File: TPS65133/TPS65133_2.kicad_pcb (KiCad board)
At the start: 2 copper layers, 19.8 x 40.1 mm, 14 parts, among them IC1 TPS65133DPDR, J1 Conn_02x03_Odd_Even, J2 Conn_02x03_Odd_Even, J3 Conn_02x03_Odd_Even

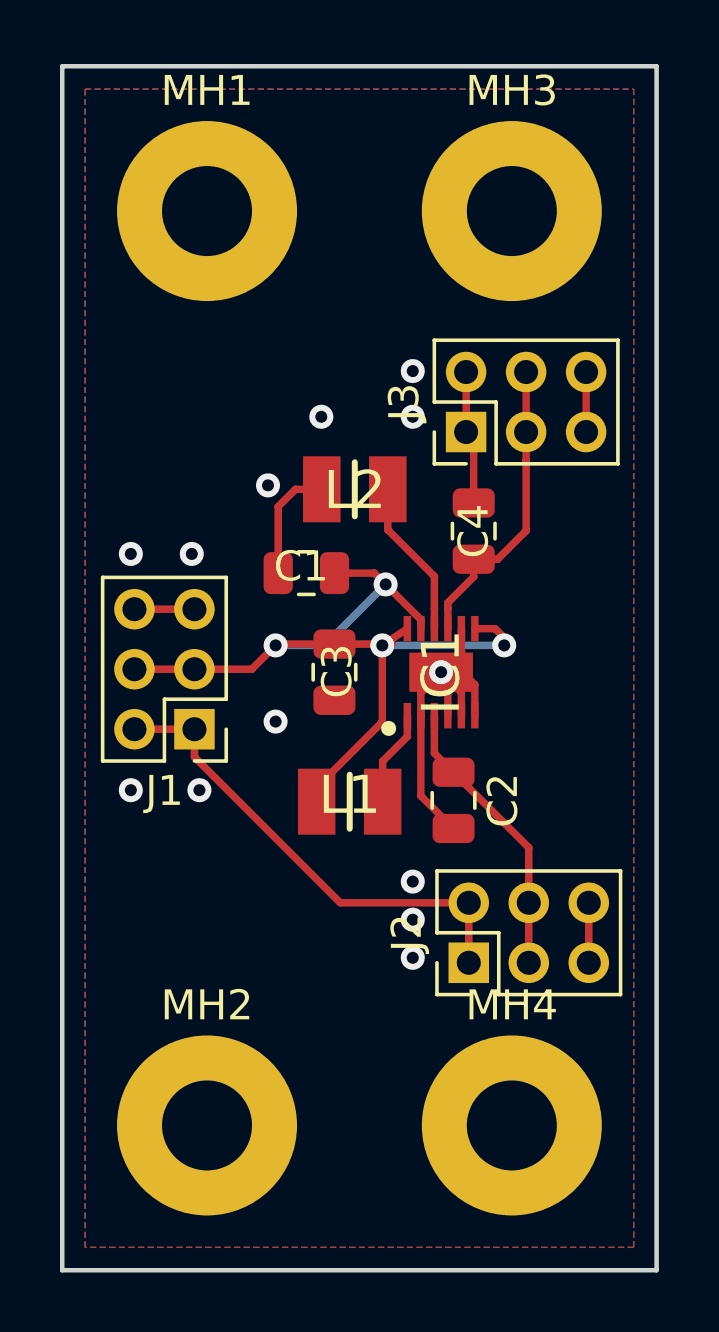
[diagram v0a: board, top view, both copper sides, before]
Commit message: TPS65133
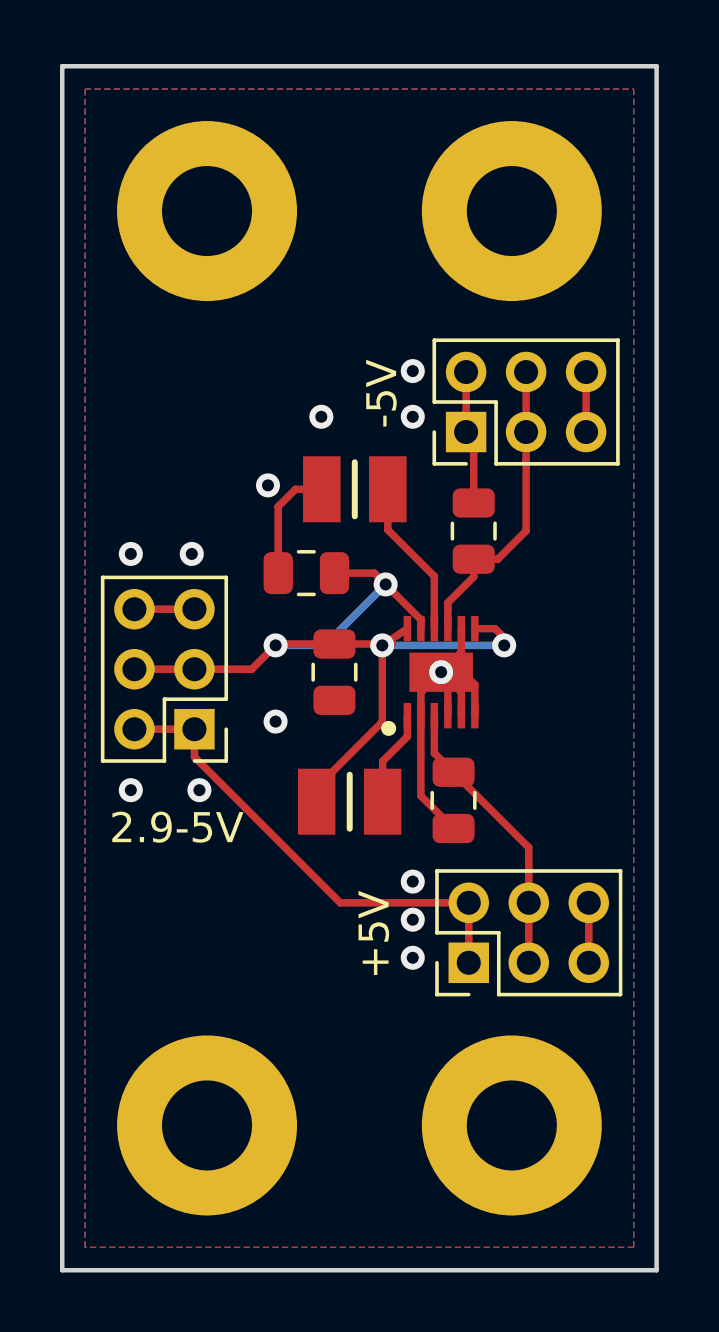
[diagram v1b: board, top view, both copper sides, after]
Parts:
- removed C1: 100nF, Capacitor_SMD:C_0805_2012Metric
- added ?: 100nF, Capacitor_SMD:C_0805_2012Metric, F.Cu at (115.1, 75.6)
- renumbered J2 to +5V, J3 to -5V, J1 to 2.9-5V, MH3 to ?, MH4 to ?, C2 to ?, C3 to ?, C4 to ?, IC1 to ?, L1 to ?, L2 to ?, MH1 to ?, MH2 to ?
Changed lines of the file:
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@@
     (38 B.Mask user)
     (39 F.Mask user)
-    (40 Dwgs.User user hide)
+    (40 Dwgs.User user)
     (41 Cmts.User user)
     (42 Eco1.User user)
@@
     (tags capacitor)
     (attr smd)
-    (fp_text reference C1 (at 0.173907 0.219262) (layer F.SilkS)
+    (fp_text reference "" (at 2.548321 1.400848 90) (layer F.SilkS)
       (effects (font (size 1 1) (thickness 0.15)))
     )
@@
     (tags capacitor)
     (attr smd)
-    (fp_text reference C2 (at 0 -1.65 270) (layer F.SilkS)
+    (fp_text reference "" (at 0 -1.65 270) (layer F.SilkS)
       (effects (font (size 1 1) (thickness 0.15)))
     )
@@
     (tags capacitor)
     (attr smd)
-    (fp_text reference C3 (at -0.034738 -0.095407 270) (layer F.SilkS)
+    (fp_text reference "" (at -0.034738 -0.095407 270) (layer F.SilkS)
       (effects (font (size 1 1) (thickness 0.15)))
     )
@@
     (tags capacitor)
     (attr smd)
-    (fp_text reference C4 (at 0 0 90) (layer F.SilkS)
+    (fp_text reference "" (at 0 0 90) (layer F.SilkS)
       (effects (font (size 1 1) (thickness 0.15)))
     )
@@
     (tags "Integrated Circuit")
     (attr smd)
-    (fp_text reference IC1 (at 0 0 90) (layer F.SilkS)
+    (fp_text reference "" (at 0 0 90) (layer F.SilkS)
       (effects (font (size 1.27 1.27) (thickness 0.254)))
     )
@@
     (descr "Through hole straight pin header, 2x03, 2.00mm pitch, double rows")
     (tags "Through hole pin header THT 2x03 2.00mm double row")
-    (fp_text reference J1 (at 1 -2.06 180) (layer F.SilkS)
+    (fp_text reference 2.9-5V (at 0.596414 -3.302 180) (layer F.SilkS)
       (effects (font (size 1 1) (thickness 0.15)))
     )
@@
     (descr "Through hole straight pin header, 2x03, 2.00mm pitch, double rows")
     (tags "Through hole pin header THT 2x03 2.00mm double row")
-    (fp_text reference J2 (at 1 -2.06 90) (layer F.SilkS)
+    (fp_text reference +5V (at 0.927586 -3.136414 90) (layer F.SilkS)
       (effects (font (size 1 1) (thickness 0.15)))
     )
@@
     (descr "Through hole straight pin header, 2x03, 2.00mm pitch, double rows")
     (tags "Through hole pin header THT 2x03 2.00mm double row")
-    (fp_text reference J3 (at 1 -2.06 90) (layer F.SilkS)
+    (fp_text reference -5V (at 1.27 -2.794 90) (layer F.SilkS)
       (effects (font (size 1 1) (thickness 0.15)))
     )
@@
     (tags Inductor)
     (attr smd)
-    (fp_text reference L1 (at 0 0.219262) (layer F.SilkS)
+    (fp_text reference "" (at 0 0.219262) (layer F.SilkS)
       (effects (font (size 1.27 1.27) (thickness 0.254)))
     )
@@
     (tags Inductor)
     (attr smd)
-    (fp_text reference L2 (at 0 -0.034738) (layer F.SilkS)
+    (fp_text reference "" (at 0 -0.034738) (layer F.SilkS)
       (effects (font (size 1.27 1.27) (thickness 0.254)))
     )
@@
     (tags "mounting hole 3mm")
     (attr virtual)
-    (fp_text reference MH1 (at 0 -4) (layer F.SilkS)
+    (fp_text reference "" (at 0 -4) (layer F.SilkS)
       (effects (font (size 1 1) (thickness 0.15)))
     )
@@
     (tags "mounting hole 3mm")
     (attr virtual)
-    (fp_text reference MH2 (at 0 -4) (layer F.SilkS)
+    (fp_text reference "" (at 0 -4) (layer F.SilkS)
       (effects (font (size 1 1) (thickness 0.15)))
     )
@@
     (tags "mounting hole 3mm")
     (attr virtual)
-    (fp_text reference MH3 (at 0 -4) (layer F.SilkS)
+    (fp_text reference "" (at 0 -4) (layer F.SilkS)
       (effects (font (size 1 1) (thickness 0.15)))
     )
@@
     (tags "mounting hole 3mm")
     (attr virtual)
-    (fp_text reference MH4 (at 0 -4) (layer F.SilkS)
-      (effects (font (size 1 1) (thickness 0.15)))
-    )
+    (fp_text reference "" (at 0 -4) (layer F.SilkS)
+      (effects (font (size 1 1) (thickness 0.15)))
+    )
